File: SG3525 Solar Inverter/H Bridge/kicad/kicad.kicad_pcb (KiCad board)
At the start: 2 copper layers, 106.7 x 75.3 mm, 89 parts, among them J1 Screw_Terminal_01x01, J2 Screw_Terminal_01x02, J3 Screw_Terminal_01x02, J4 Screw_Terminal_01x02, J5 Screw_Terminal_01x01, J6 Conn_01x02_Socket, Q1 IRF740, Q2 IRF740, Q3 S8050, Q4 S8050, Q5 IRF740, Q6 IRF740, Q7 BC547, U1 SG3525, U2 PC817, U3 LM358, U4 PC817

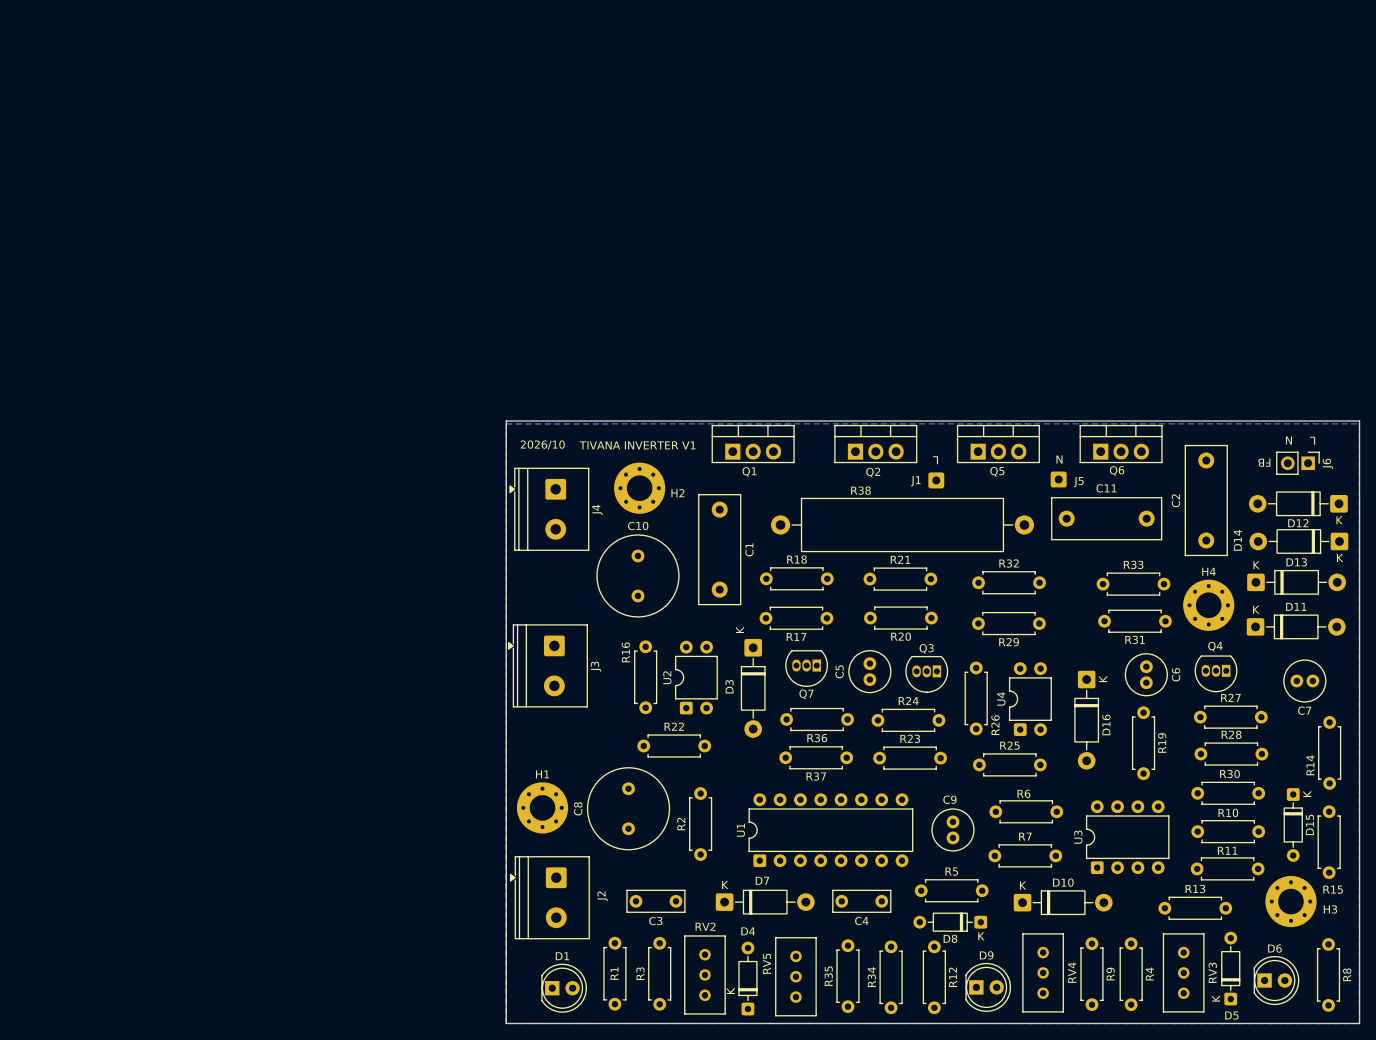
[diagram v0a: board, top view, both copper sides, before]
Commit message: WORKING ON H Bridge kicad
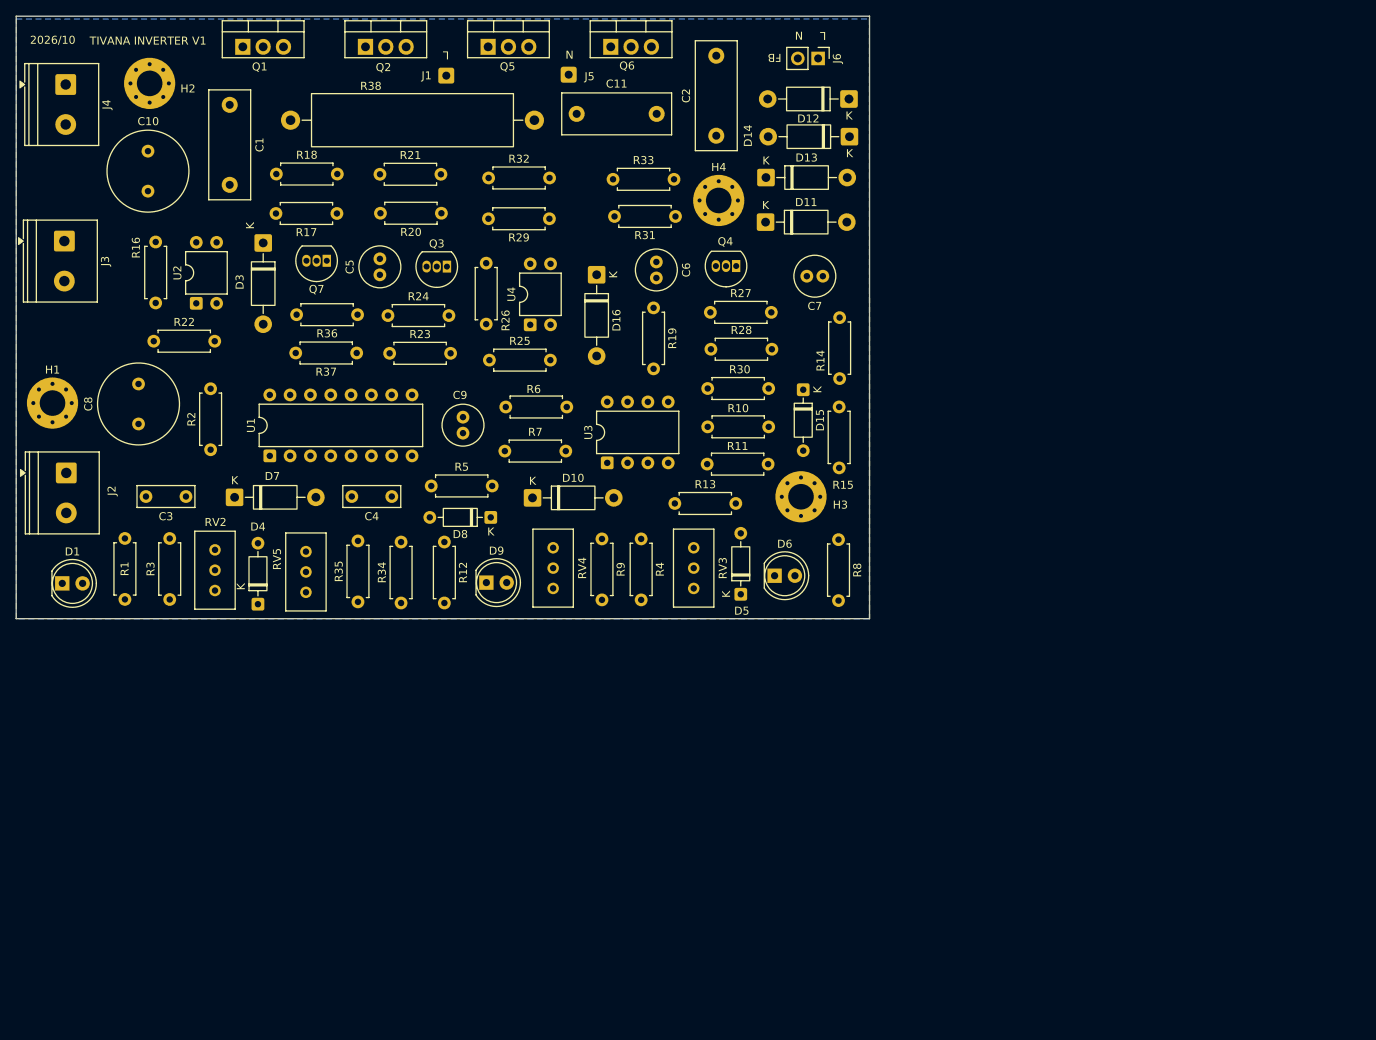
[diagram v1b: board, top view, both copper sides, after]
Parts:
- moved C1 79.4 mm to (49.5, 33.2)
- moved C2 79.4 mm to (110.4, 37.1)
- moved C3 79.4 mm to (44.1, 82.2)
- moved C4 79.4 mm to (69.8, 82.2)
- moved C5 79.4 mm to (68.3, 54.5)
- moved C6 79.4 mm to (102.9, 52.9)
- moved C7 79.4 mm to (123.7, 54.6)
- moved C8 79.4 mm to (38.1, 73.1)
- moved C9 79.4 mm to (78.7, 74.2)
- moved D11 79.4 mm to (116.5, 47.9)
- moved D12 79.4 mm to (127.0, 32.5)
- moved D13 79.4 mm to (116.6, 42.3)
- moved D14 79.4 mm to (127.0, 37.2)
- moved D15 79.4 mm to (121.2, 68.8)
- moved D3 79.4 mm to (53.7, 50.5)
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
